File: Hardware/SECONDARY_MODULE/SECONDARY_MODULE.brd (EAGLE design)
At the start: 100 x 69.8 mm, 19 parts

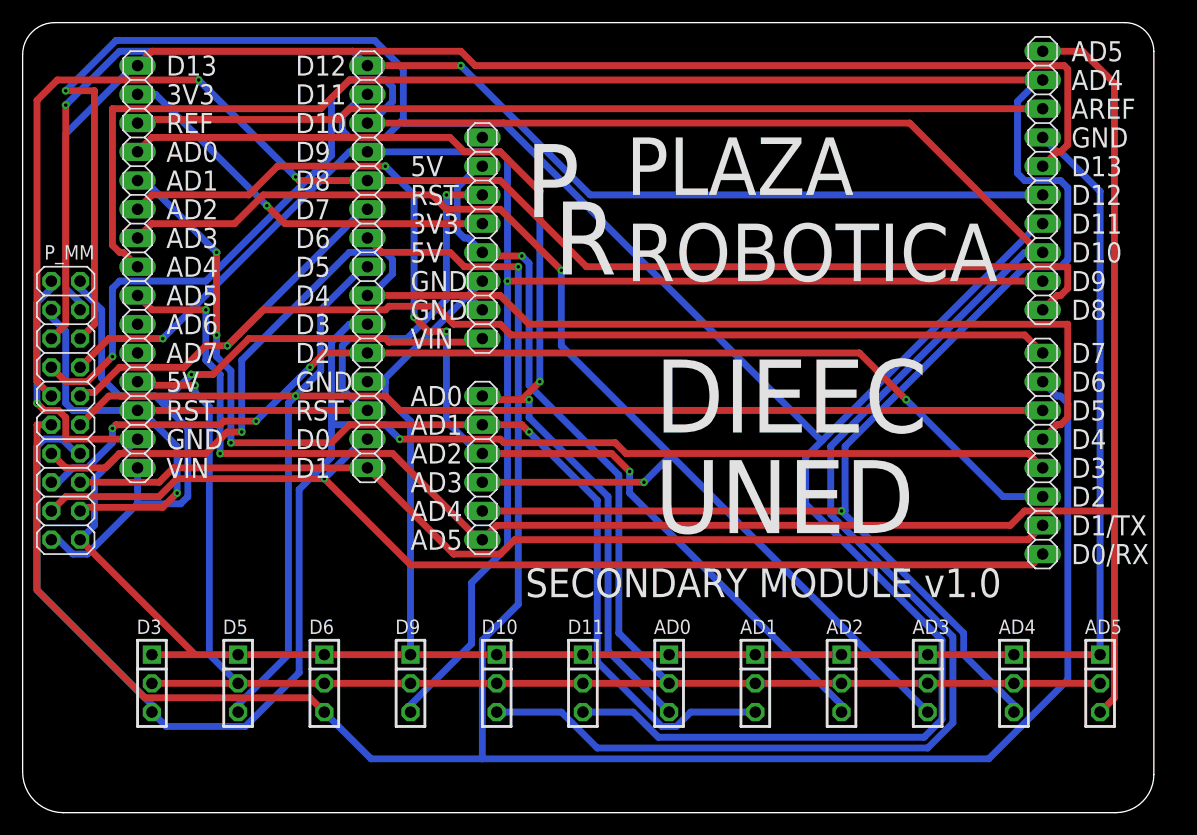
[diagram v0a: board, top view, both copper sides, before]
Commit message: Add files via upload
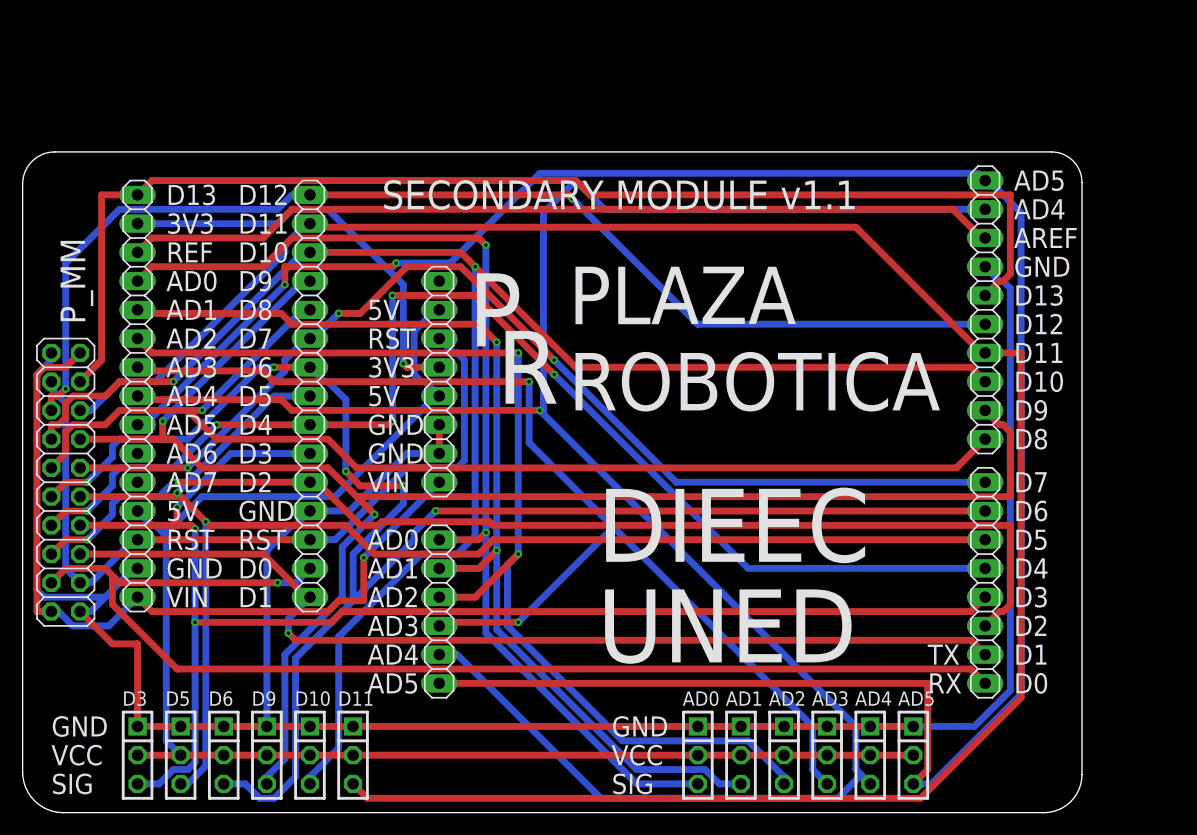
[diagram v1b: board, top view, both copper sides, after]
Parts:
- moved D11 21.3 mm to (29.2, 5.08)
- moved AD5 17.7 mm to (78.7, 5.08)
- moved D10 17.7 mm to (25.4, 5.08)
- moved D9 14.2 mm to (21.6, 5.08)
- moved AD4 14.2 mm to (74.9, 5.08)
- moved SA_A 13.3 mm to (36.8, 17.8)
- moved SA_P 13.3 mm to (36.8, 38.1)
- moved NANO_D 12.5 mm to (25.4, 36.8)
- moved SA_D1 12.5 mm to (85.1, 20.3)
- moved SA_D2 12.5 mm to (85.1, 44.5)
- moved NANO_A 11.4 mm to (10.2, 36.8)
- moved AD3 10.9 mm to (71.1, 5.08)
- moved D6 10.9 mm to (17.8, 5.08)
- moved D5 8.13 mm to (14.0, 5.08)
- moved AD2 8.13 mm to (67.3, 5.08)
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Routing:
- net D10: track 214.5 -> 149.2 mm, vias 1 -> 2
- net D6: track 202.7 -> 141.2 mm, vias 1 -> 5
- net VCC: track 173.6 -> 131.1 mm, vias 2 -> 0
- net AD5: track 166.9 -> 198.1 mm
- net D8: track 130.3 -> 103.4 mm, vias 2 -> 1
- net AD4: track 207.4 -> 183.4 mm
- net D11: track 212.6 -> 188.9 mm, vias 1 -> 0
- net D3: track 146.5 -> 122.9 mm, vias 1 -> 3
- net GND: track 222.3 -> 201.8 mm, vias 1 -> 0
- net RST: track 84.0 -> 69.2 mm, vias 2 -> 0
- net D4: track 121.1 -> 108.0 mm, vias 1 -> 5
- net D12: track 114.8 -> 102.4 mm
- net D7: track 107.5 -> 95.8 mm, vias 1 -> 3
- net AD3: track 111.9 -> 100.6 mm
- net D13: track 118.0 -> 108.7 mm
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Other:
- board size 100 x 69.8 mm -> 93.7 x 58.4 mm
- board text added: "RX"
- board text added: "SECONDARY MODULE v1.1"
- board text added: "SIG"
- board text added: "TX"
- board text added: "VCC"
- board text removed: "D0/RX"
- board text removed: "D1/TX"
- board text removed: "SECONDARY MODULE v1.0"
